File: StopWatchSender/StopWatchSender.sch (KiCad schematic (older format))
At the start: 11 parts, among them IC1 ArduinoProMini, J1 Conn_01x02_Male, SW1 SW_SPST, SW2 SW_SPST, SW3 SW_SPST, SW4 SW_SPST, SW5 SW_SPST, U1 NRF24L01

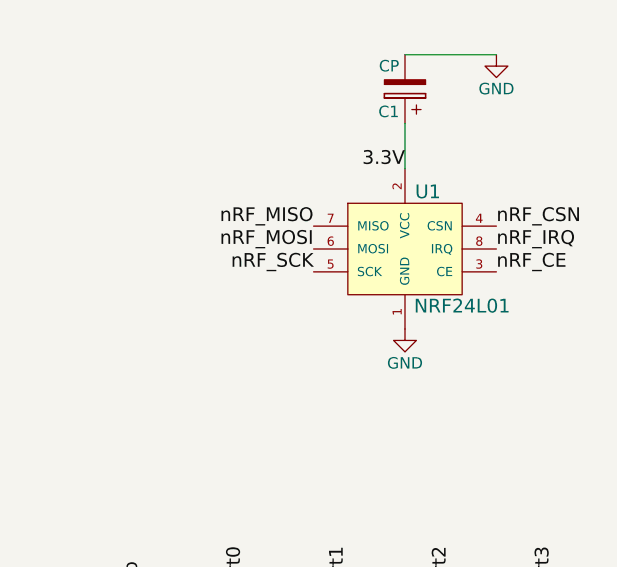
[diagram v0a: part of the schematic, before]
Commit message: KiCad PCB update
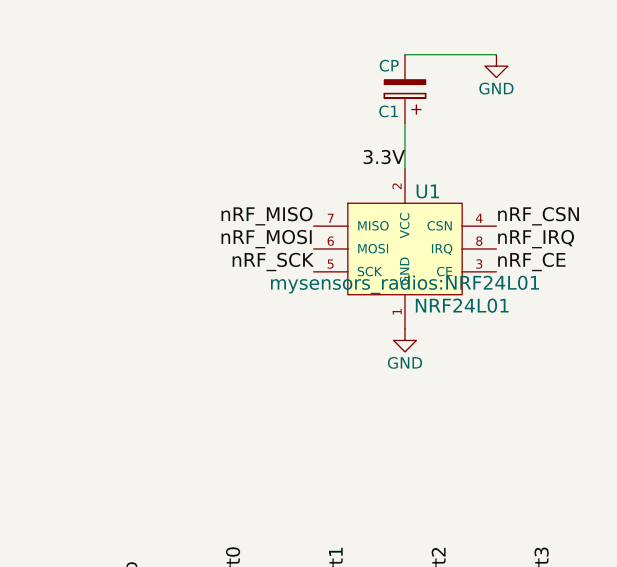
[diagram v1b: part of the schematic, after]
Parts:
- C1: footprint (none) -> Capacitors_THT:CP_Radial_D4.0mm_P1.50mm
- IC1: footprint mysensors_arduino:pro_mini_china -> mysensors_arduino:pro_mini
- U1: footprint (none) -> mysensors_radios:NRF24L01
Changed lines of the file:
@@
 F 0 "IC1" H 1750 3750 40  0000 L BNN
 F 1 "ArduinoProMini" H 2900 1100 40  0000 L BNN
-F 2 "mysensors_arduino:pro_mini_china" H 2500 2500 30  0001 C CIN
+F 2 "mysensors_arduino:pro_mini" H 2500 2500 30  0001 C CIN
 F 3 "" H 2500 2500 60  0000 C CNN
 	1    2500 2500
@@
 F 0 "U1" H 7350 2950 60  0000 C CNN
 F 1 "NRF24L01" H 7500 2450 60  0000 C CNN
-F 2 "" H 7250 2550 60  0000 C CNN
+F 2 "mysensors_radios:NRF24L01" H 7250 2550 60  0000 C CNN
 F 3 "" H 7250 2550 60  0000 C CNN
 	1    7250 2700
@@
 F 0 "C1" H 7275 2100 50  0000 L CNN
 F 1 "CP" H 7275 1900 50  0000 L CNN
-F 2 "" H 7288 1850 50  0001 C CNN
+F 2 "Capacitors_THT:CP_Radial_D4.0mm_P1.50mm" H 7288 1850 50  0001 C CNN
 F 3 "" H 7250 2000 50  0001 C CNN
 	1    7250 2000
